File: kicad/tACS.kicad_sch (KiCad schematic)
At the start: 24 parts, among them J1 +35V, J2 -35V, J3 GND/ELETRODO(-), J4 METER(+), J5 ENTRADA SINAL, J6 METER(-), J7 ELETRODO(+), Q1 TIP42C, Q2 TIP41C, Q3 2N5401, Q4 2N5551, U1 LM741, U2 LM741

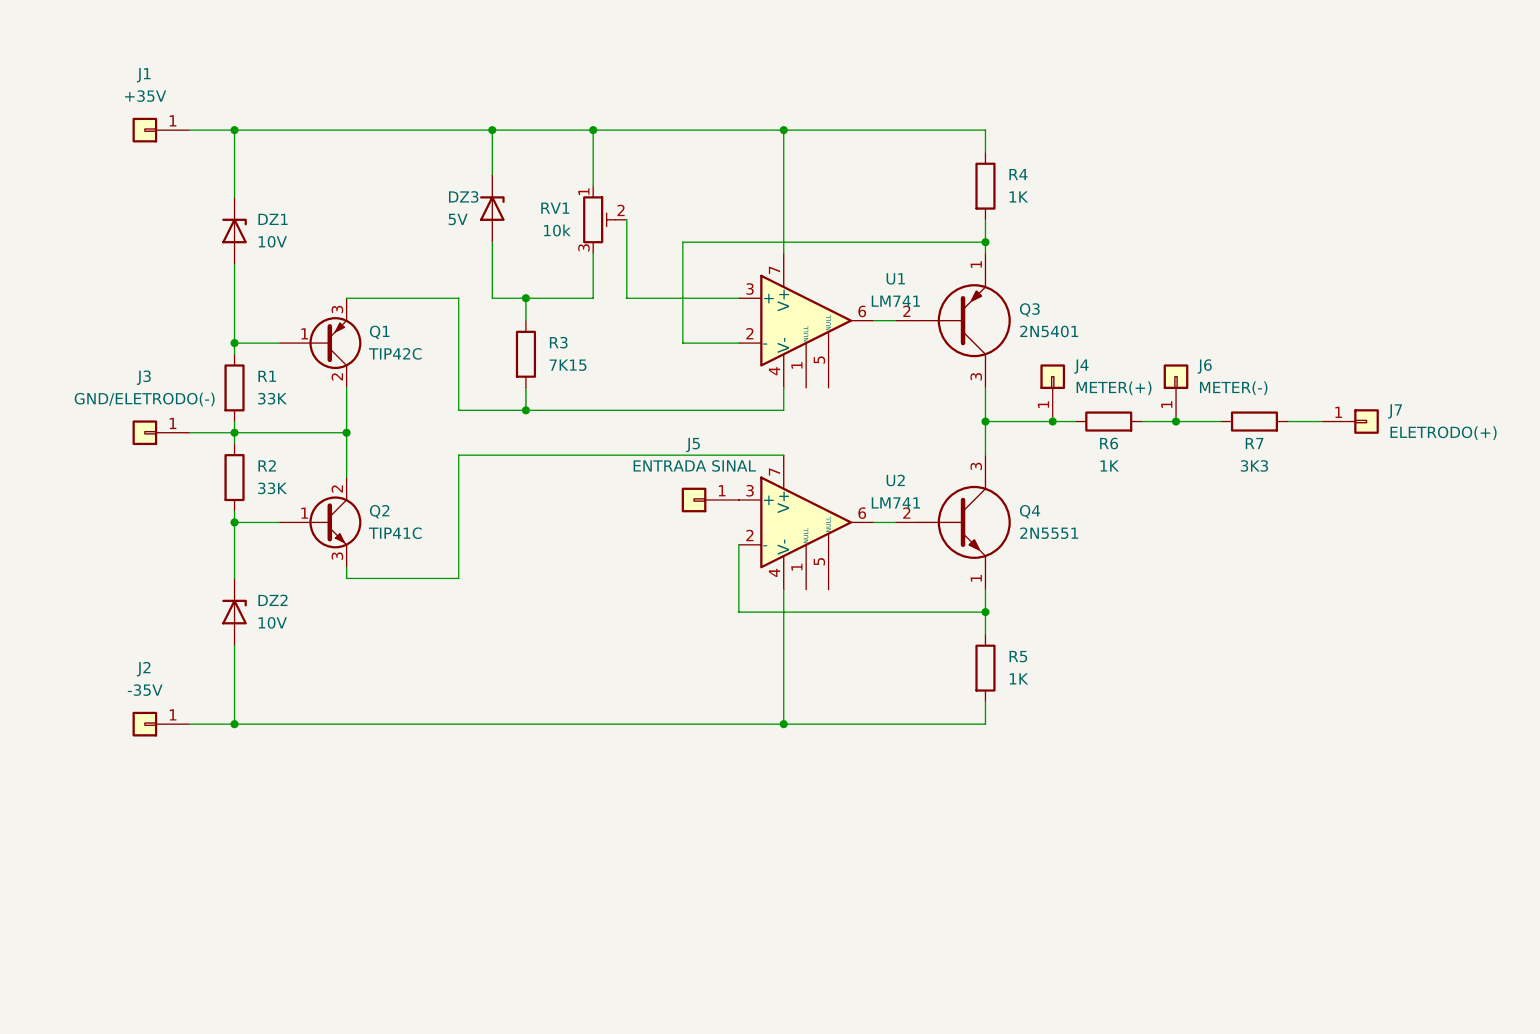
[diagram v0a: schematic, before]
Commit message: Add files via upload
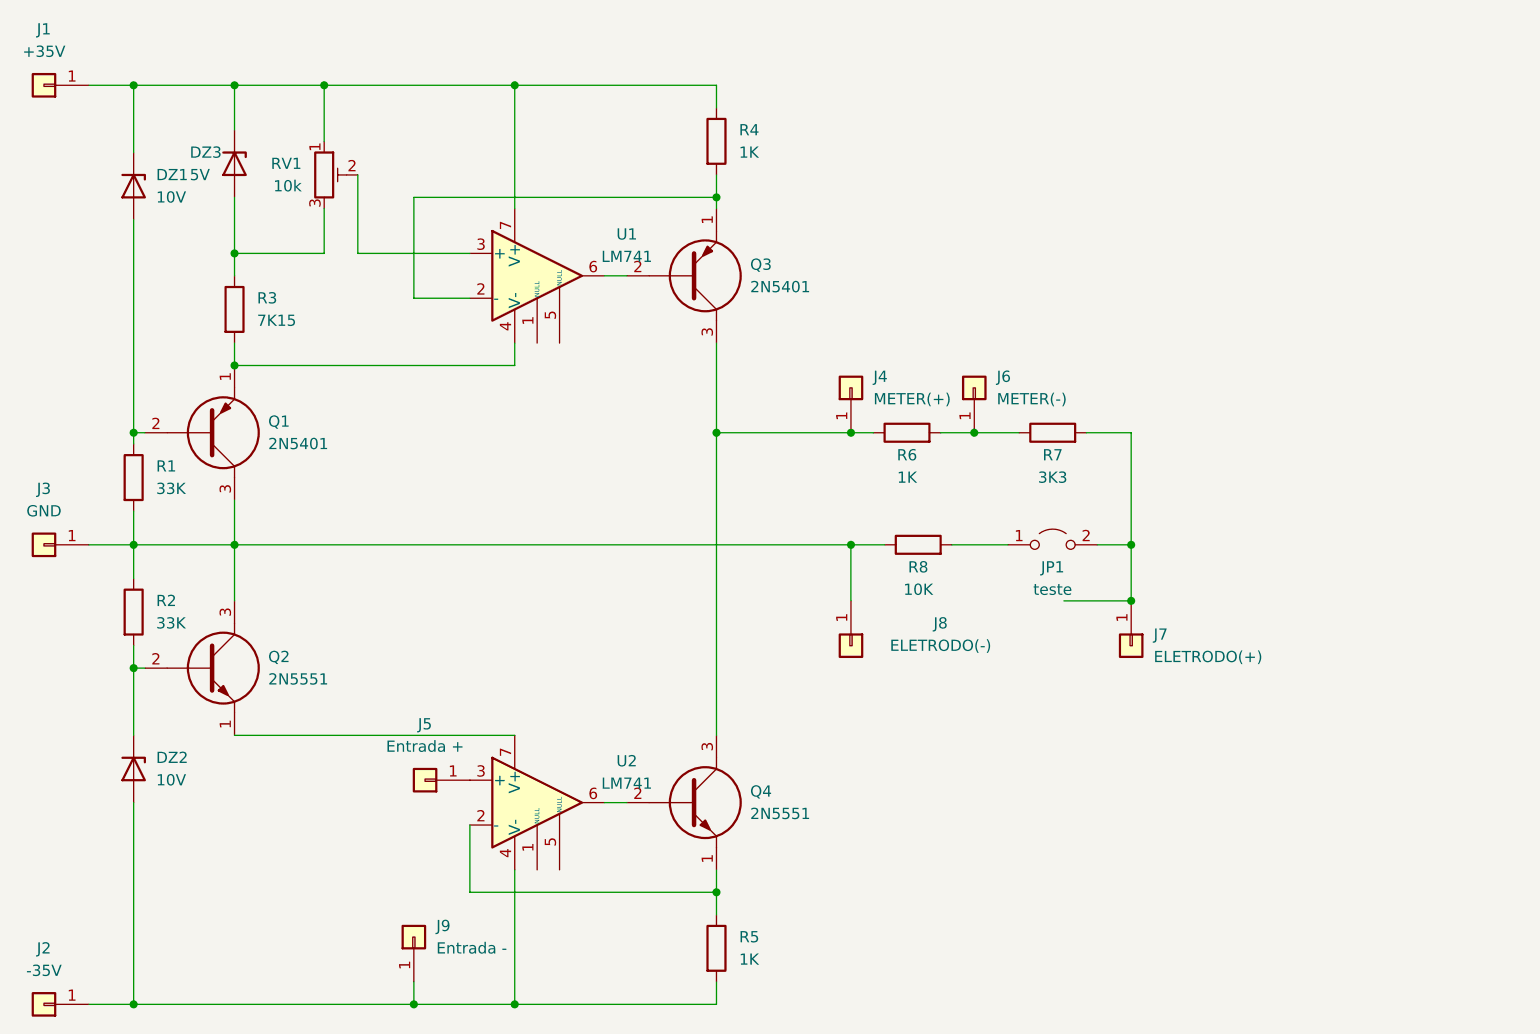
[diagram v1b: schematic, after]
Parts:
- removed Q1: TIP42C, Package_TO_SOT_THT:TO-220-3_Vertical, symbol Transistor_BJT:TIP42C
- removed Q2: TIP41C, Package_TO_SOT_THT:TO-220-3_Vertical, symbol Transistor_BJT:TIP41C
- added J8: ELETRODO(-), tACS:Pin_D0.9mm_L10.0mm_W2.4mm_FlatFork, symbol Connector_Generic:Conn_01x01
- added J9: Entrada -, tACS:Pin_D0.9mm_L10.0mm_W2.4mm_FlatFork, symbol Connector_Generic:Conn_01x01
- added JP1: teste, tACS:PinHeader_1x02_P2.54mm_Vertical, symbol Jumper:Jumper_2_Open
- added Q1: 2N5401, tACS:TO-92L_Wide, symbol SamacSys_Parts:2N5401
- added Q2: 2N5551, tACS:TO-92L_Wide, symbol SamacSys_Parts:2N5551
- added R8: 10K, tACS:R_Axial_DIN0204_L3.6mm_D1.6mm_P2.54mm_Vertical, symbol Device:R
- DZ1, DZ2, DZ3: footprint Diode_THT:D_DO-41_SOD81_P7.62mm_Horizontal -> tACS:D_DO-34_SOD68_P2.54mm_Vertical_AnodeUp
- J1, J2, J4, J6, J7: footprint Connector_Pin:Pin_D0.7mm_L6.5mm_W1.8mm_FlatFork -> tACS:Pin_D0.9mm_L10.0mm_W2.4mm_FlatFork
- J3: value GND/ELETRODO(-) -> GND; footprint Connector_Pin:Pin_D0.7mm_L6.5mm_W1.8mm_FlatFork -> tACS:Pin_D0.9mm_L10.0mm_W2.4mm_FlatFork
- J5: value ENTRADA SINAL -> Entrada +; footprint Connector_Pin:Pin_D0.7mm_L6.5mm_W1.8mm_FlatFork -> tACS:Pin_D0.9mm_L10.0mm_W2.4mm_FlatFork
- Q3, Q4: footprint Package_TO_SOT_THT:TO-92 -> tACS:TO-92L_Wide
- R1, R2, R3, R4, R6, R7: footprint Resistor_THT:R_Axial_DIN0204_L3.6mm_D1.6mm_P7.62mm_Horizontal -> tACS:R_Axial_DIN0204_L3.6mm_D1.6mm_P2.54mm_Vertical
- R5: footprint Resistor_THT:R_Axial_DIN0204_L3.6mm_D1.6mm_P5.08mm_Vertical -> tACS:R_Axial_DIN0204_L3.6mm_D1.6mm_P2.54mm_Vertical
- RV1: footprint Potentiometer_THT:Potentiometer_Bourns_3296W_Vertical -> tACS:Potentiometer_Bourns_3296W_Vertical
- U1: footprint Package_DIP:DIP-8_W7.62mm_LongPads -> tACS:DIP-8_W7.62mm_LongPads
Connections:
- net at J3.1 (Pin_1), R1.2, R2.1: now also J8.1 (Pin_1), Q1.3, Q2.3, R8.1
- net at DZ2.1 (K), R2.2: now also Q2.2
- net at U2.7 (V+): now also Q2.1
- net at DZ1.2 (A), R1.1: now also Q1.2
- net at R3.2, U1.4 (V-): now also Q1.1
- net at J7.1 (Pin_1), R7.2: now also JP1.2 (B)
- net at DZ2.2 (A), J2.1 (Pin_1), R5.2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: now also J9.1 (Pin_1)
- new net: JP1.1 (A), R8.2
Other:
- moved on the sheet: DZ1, DZ2, DZ3, J1, J2, J3, J4, J5, J6, J7, Q3, Q4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
